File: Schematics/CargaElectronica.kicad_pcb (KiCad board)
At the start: 2 copper layers, 88 x 94.2 mm, 57 parts, among them J1 Voltage_test, J2 Voltage_IN, J3 FAN_OUTPUT, Q1 IRFP460, Q2 Q_NMOS_GSD, SW1 Rotary_Encoder_Switch, SW2 Btn.OK, SW3 Btn.BCK, U1 TL072, U2 Pantalla_LCD_16x2_i2c, U3 LM35-LP, U4 TL431DBZ

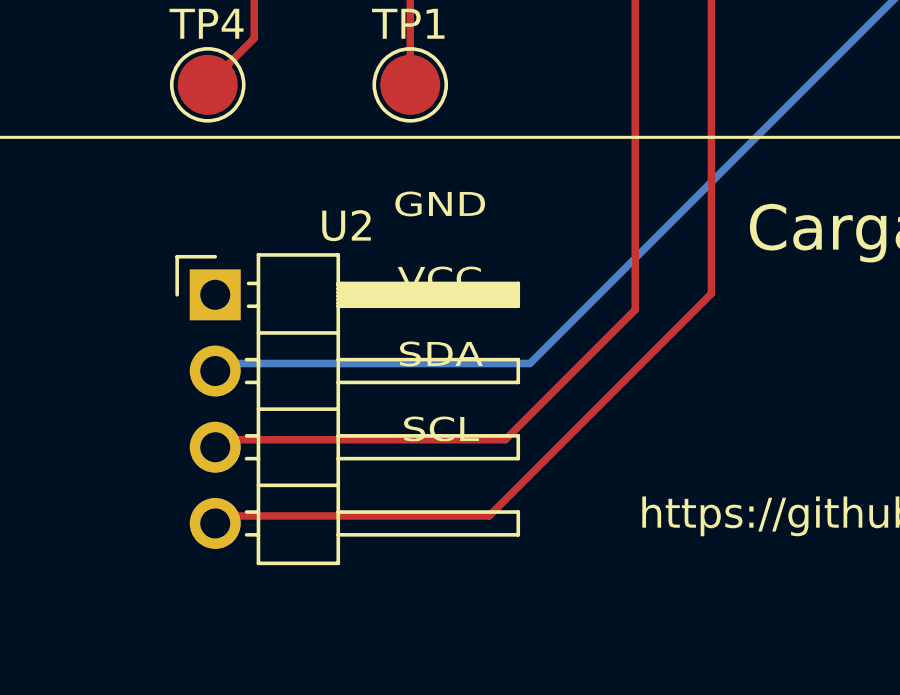
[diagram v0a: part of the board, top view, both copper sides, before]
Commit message: Fix for PCB v1 and more sourcecode
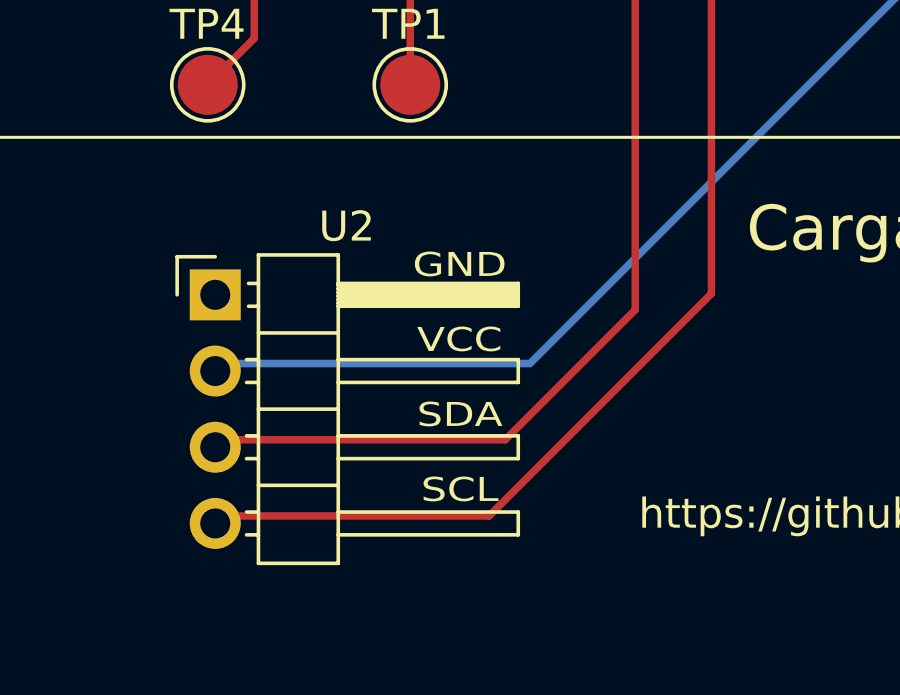
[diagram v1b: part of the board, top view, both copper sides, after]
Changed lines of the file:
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@@
     (effects (font (size 1.5 1.5) (thickness 0.3)))
   )
-  (gr_text "SCL\n" (at 116.75 104.5) (layer "F.SilkS")
+  (gr_text "SCL\n" (at 117.4 106.5) (layer "F.SilkS")
     (effects (font (size 0.8 1) (thickness 0.15)))
   )
@@
     (effects (font (size 1 1) (thickness 0.15)))
   )
-  (gr_text "VCC\n" (at 116.75 99.5) (layer "F.SilkS")
+  (gr_text "VCC\n" (at 117.4 101.5) (layer "F.SilkS")
     (effects (font (size 0.8 1) (thickness 0.15)))
   )
@@
     (effects (font (size 1 1) (thickness 0.15)))
   )
-  (gr_text "SDA" (at 116.75 102) (layer "F.SilkS")
+  (gr_text "SDA" (at 117.4 104) (layer "F.SilkS")
     (effects (font (size 0.8 1) (thickness 0.15)))
   )
@@
     (effects (font (size 1 1) (thickness 0.15)))
   )
-  (gr_text "GND" (at 116.75 97) (layer "F.SilkS")
+  (gr_text "GND" (at 117.4 99) (layer "F.SilkS")
     (effects (font (size 0.8 1) (thickness 0.15)))
   )

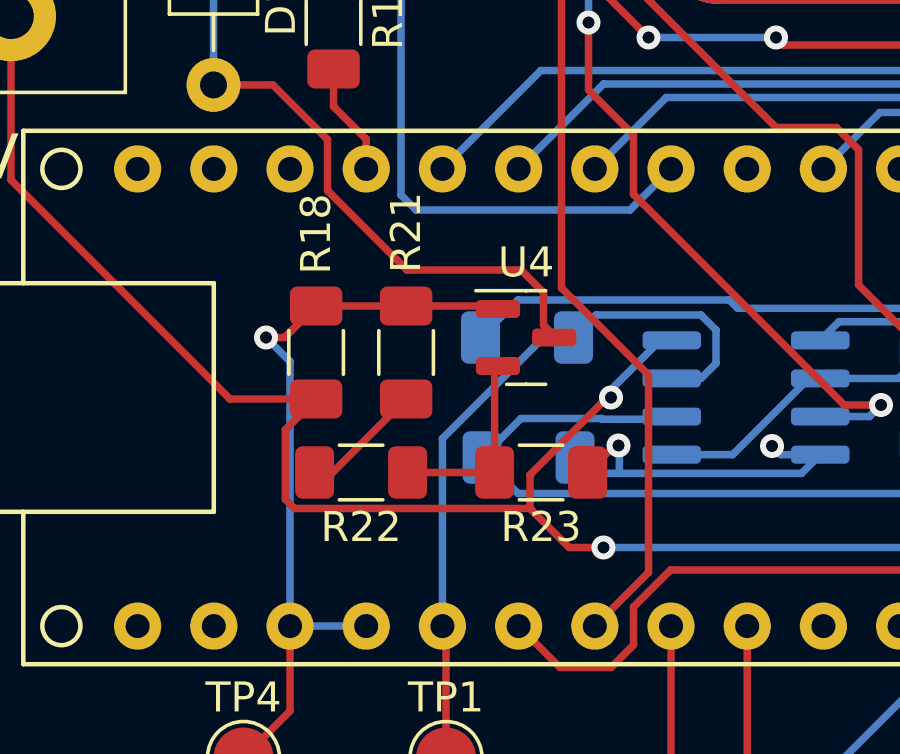
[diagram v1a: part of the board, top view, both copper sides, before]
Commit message: Version stable
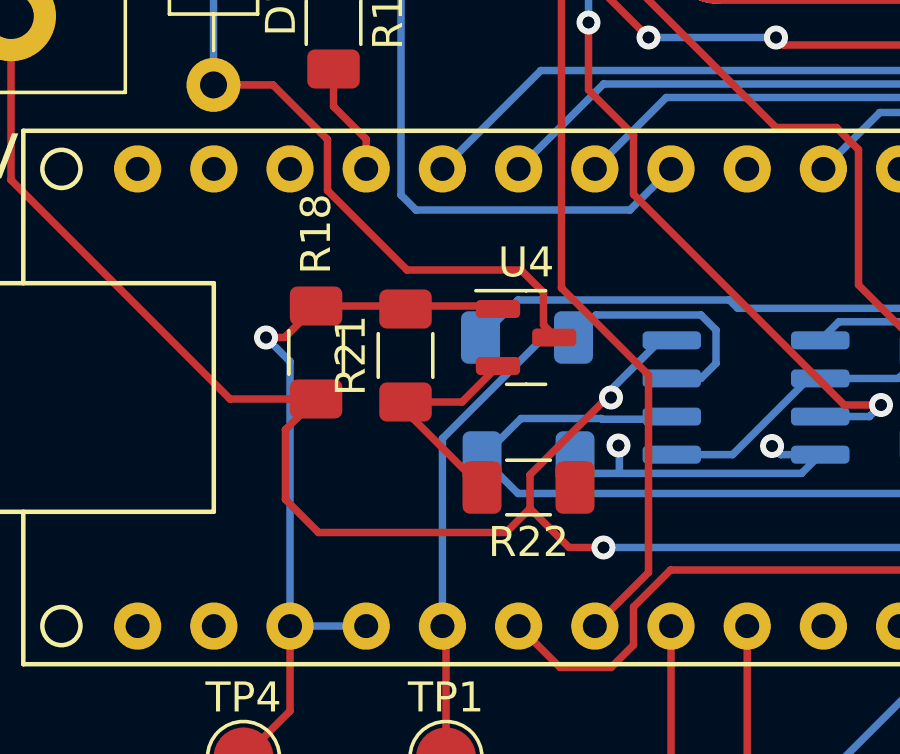
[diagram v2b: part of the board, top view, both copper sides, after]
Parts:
- removed R23: 1k5, Resistor_SMD:R_1206_3216Metric_Pad1.30x1.75mm_HandSolder
- R21: value 330 -> 1k
- R22: value 2k2 -> 1k5
- R8: value 100 -> 330
- moved R22 5.60 mm to (118.5, 84.0)
- moved R21 0.10 mm to (114.4, 79.6)
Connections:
- A1 pad 29: unconnected-(A1-Pad29) -> GND
- A1 pad 4: unconnected-(A1-Pad4) -> GND
- R21 pad 1: Net-(R21-Pad1) -> Net-(U4-Pad2)
- R22 pad 1: Net-(R22-Pad1) -> GND
- R22 pad 2: Net-(R21-Pad1) -> Net-(U4-Pad2)
- U4 pad 2: Net-(R22-Pad1) -> Net-(U4-Pad2)
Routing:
- net Net-(U4-Pad2): track 0.00 -> 7.49 mm
- net Net-(R22-Pad1): track 6.47 -> 0.00 mm
- net Net-(R21-Pad1): track 4.06 -> 0.00 mm
- net GND: track 218.6 -> 217.3 mm
- net V_IN: track 78.4 -> 79.0 mm
